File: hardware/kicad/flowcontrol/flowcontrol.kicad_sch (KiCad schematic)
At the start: 1 part, among them U3 SOL1_AND_2 SPLIT

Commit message: Schemiatic update
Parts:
- U3: footprint Package_DIP:DIP-24_W7.62mm -> Package_DIP:DIP-28_W7.62mm
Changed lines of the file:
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@@
 			)
 		)
-		(property "Footprint" "Package_DIP:DIP-24_W7.62mm"
+		(property "Footprint" "Package_DIP:DIP-28_W7.62mm"
 			(at 83.82 171.45 0)
 			(effects

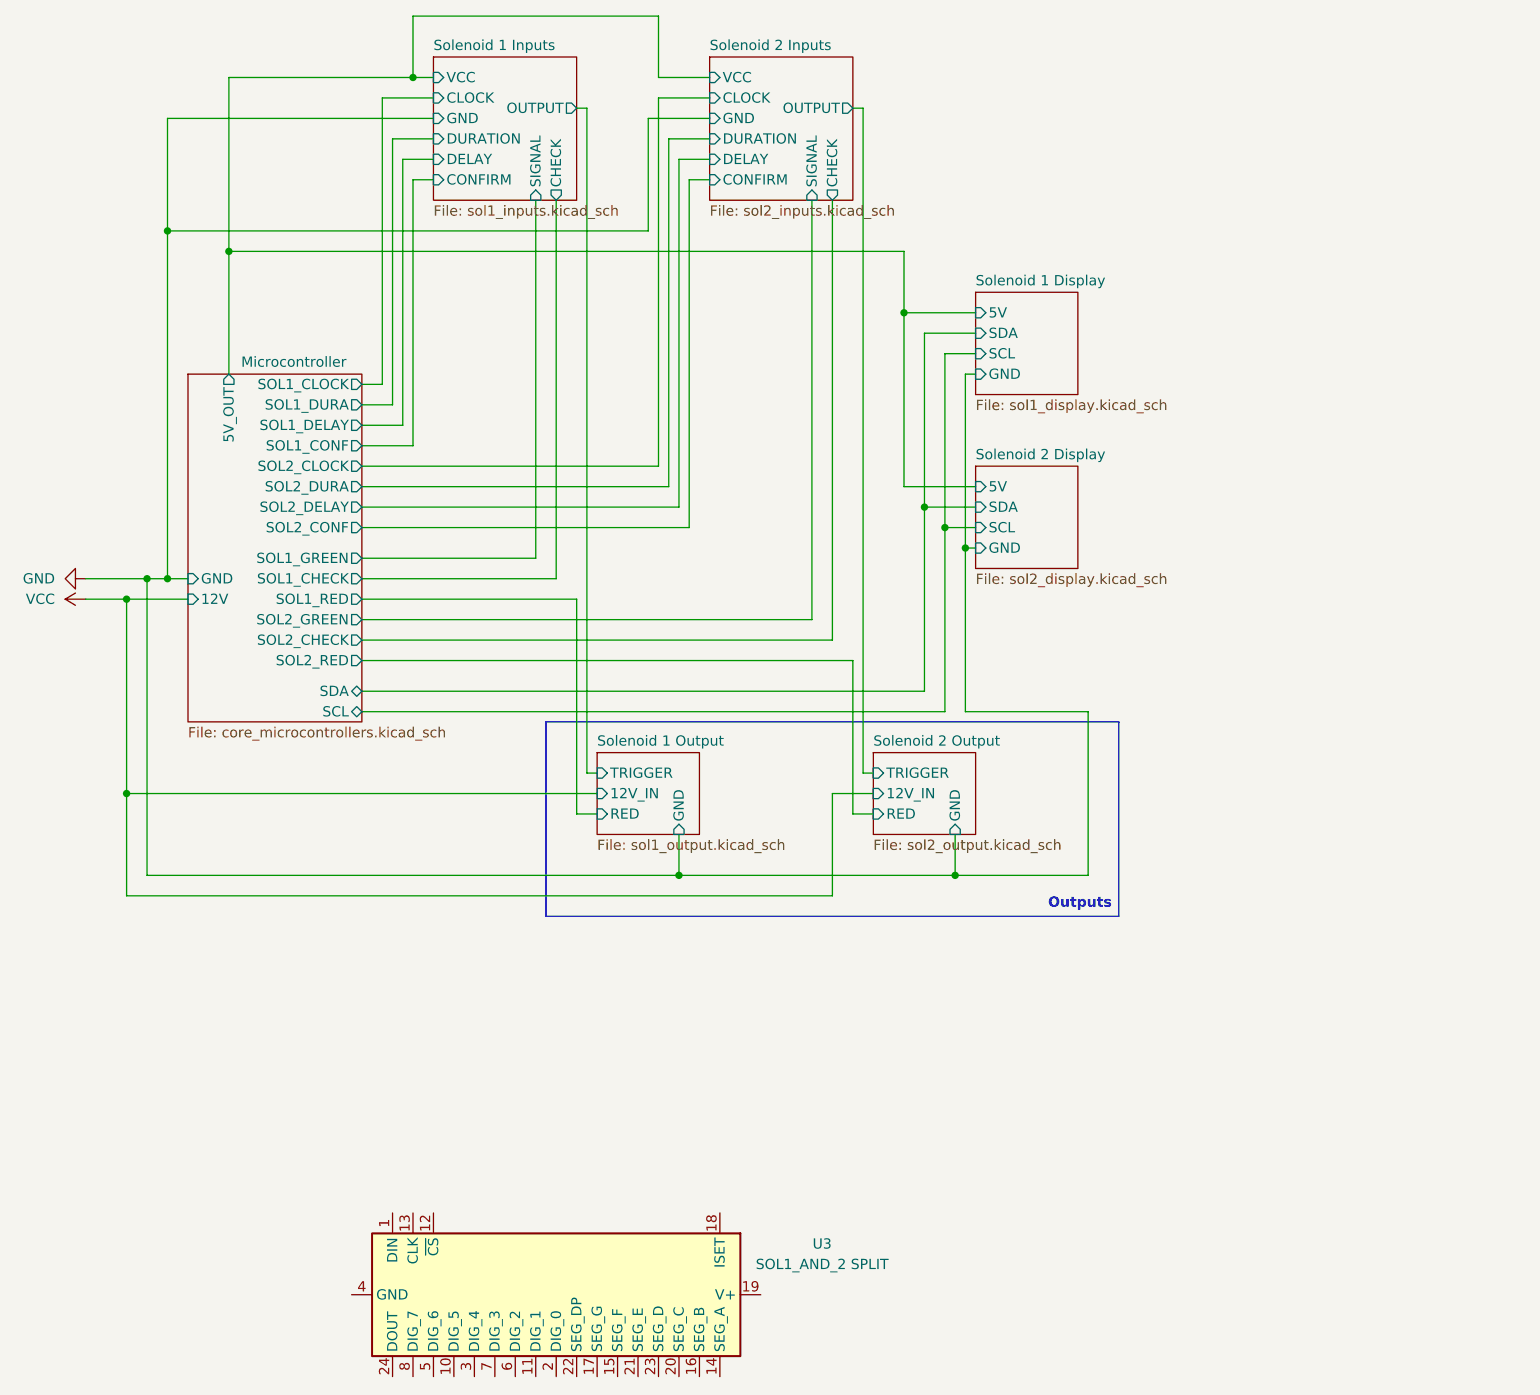
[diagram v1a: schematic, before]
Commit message: Updated KiCad schematic to final rendition
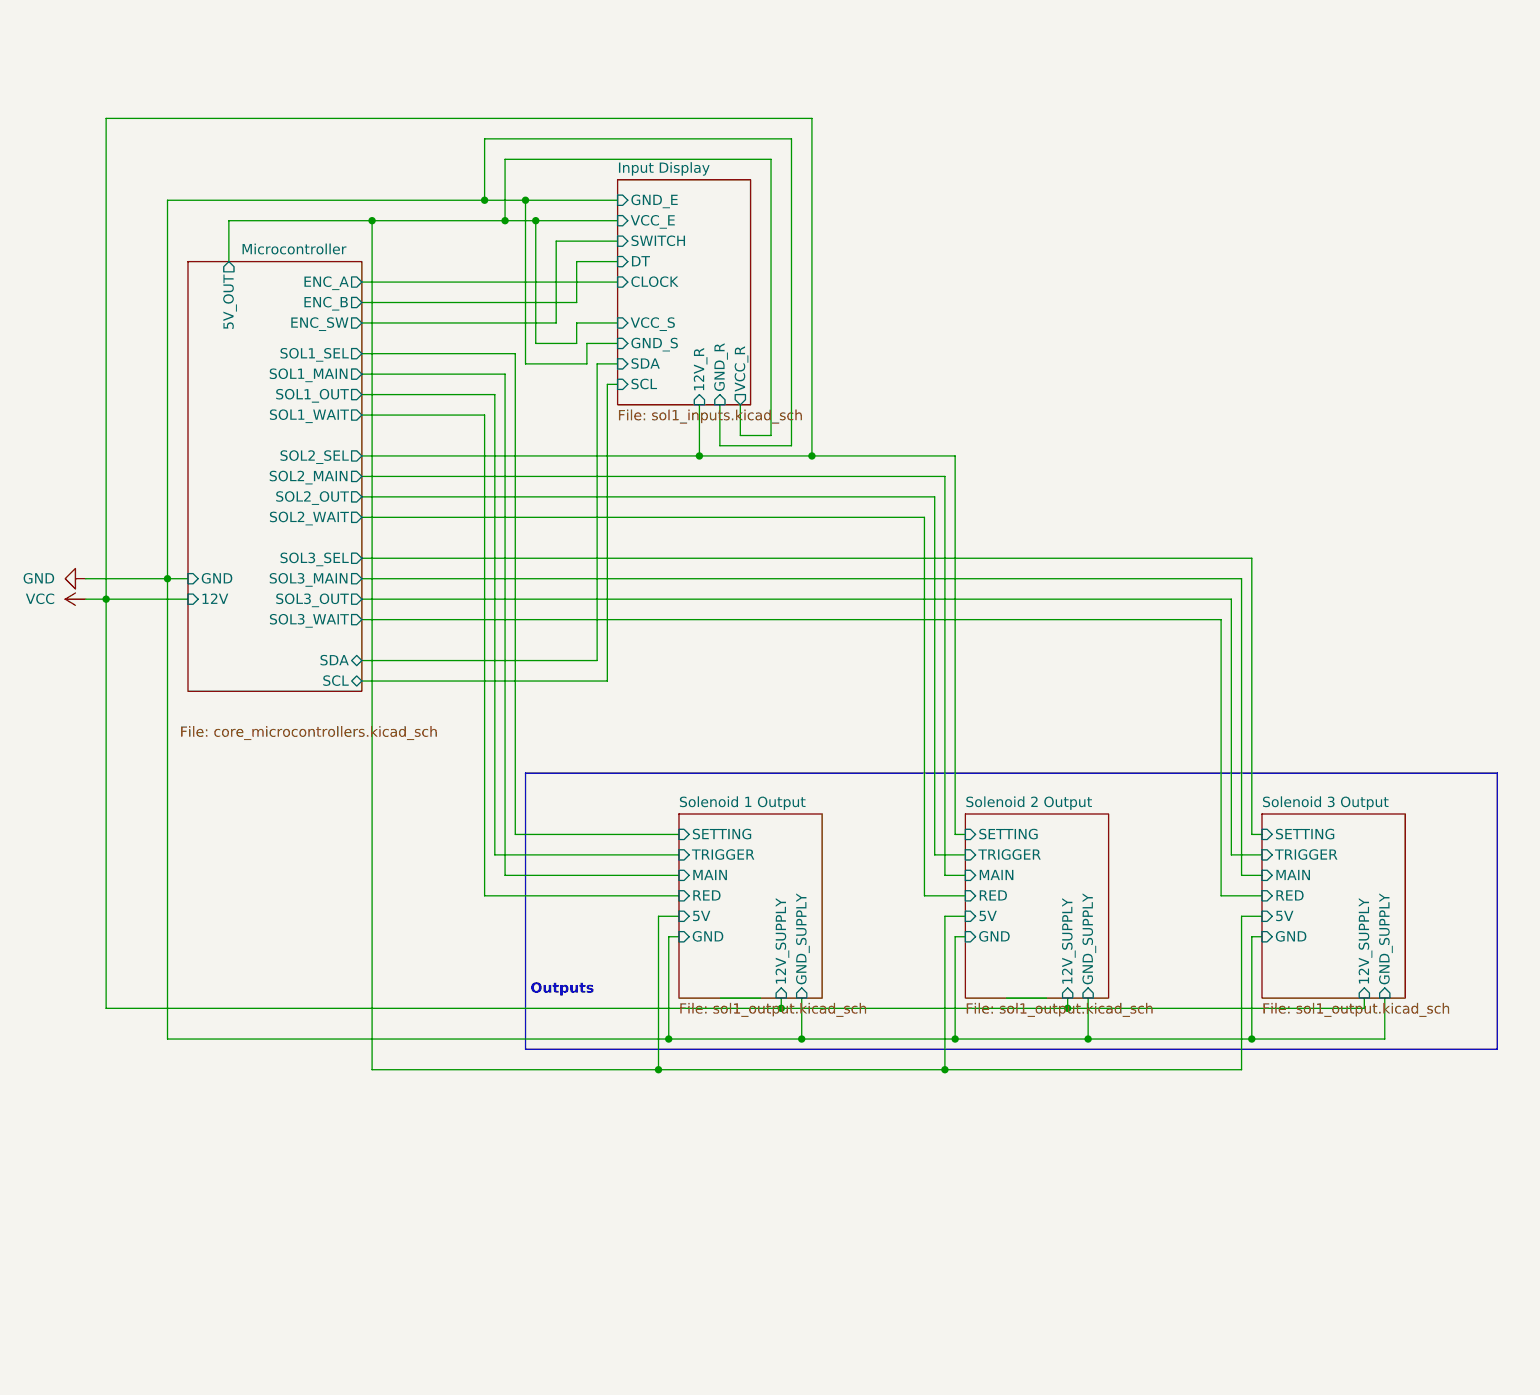
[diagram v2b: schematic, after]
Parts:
- removed U3: SOL1_AND_2 SPLIT, Package_DIP:DIP-28_W7.62mm, symbol Driver_LED:MAX7221xNG
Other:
- sheet Solenoid 1 Inputs renamed Input Display
- removed sheet Solenoid 1 Display
- removed sheet Solenoid 2 Display
- removed sheet Solenoid 2 Inputs
- added sheet Solenoid 3 Output (sol1_output.kicad_sch)
- sheet Input Display ports: added 12V_R, DT, GND_E, GND_R, GND_S, SCL, SDA, SWITCH, VCC_E, VCC_R, VCC_S; removed CHECK, CONFIRM, DELAY, DURATION, GND, OUTPUT, SIGNAL, VCC
- sheet Microcontroller ports: added ENC_A, ENC_B, ENC_SW, SOL1_MAIN, SOL1_OUT, SOL1_SEL, SOL1_WAIT, SOL2_MAIN, SOL2_OUT, SOL2_SEL, SOL2_WAIT, SOL3_MAIN, SOL3_OUT, SOL3_SEL, SOL3_WAIT; removed SOL1_CHECK, SOL1_CLOCK, SOL1_CONF, SOL1_DELAY, SOL1_DURA, SOL1_GREEN, SOL1_RED, SOL2_CHECK, SOL2_CLOCK, SOL2_CONF, SOL2_DELAY, SOL2_DURA, SOL2_GREEN, SOL2_RED
- sheet Solenoid 1 Output ports: added 12V_SUPPLY, 5V, GND_SUPPLY, MAIN, SETTING; removed 12V_IN
- sheet Solenoid 2 Output: file sol2_output.kicad_sch -> sol1_output.kicad_sch
- sheet Solenoid 2 Output ports: added 12V_SUPPLY, 5V, GND_SUPPLY, MAIN, SETTING; removed 12V_IN
